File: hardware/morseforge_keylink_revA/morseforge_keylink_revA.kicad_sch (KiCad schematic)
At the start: 28 parts, among them J1 USB_C_Receptacle_USB2.0_14P, J2 Conn_01x02_Socket, Q1 Q_NPN_BCE, SW1 SW_SPST, SW2 SW_Push, SW3 SW_Push, U1 MCP73831-2-MC, U2 LDO40LPU33RY, U3 CP2102N-Axx-xQFN20

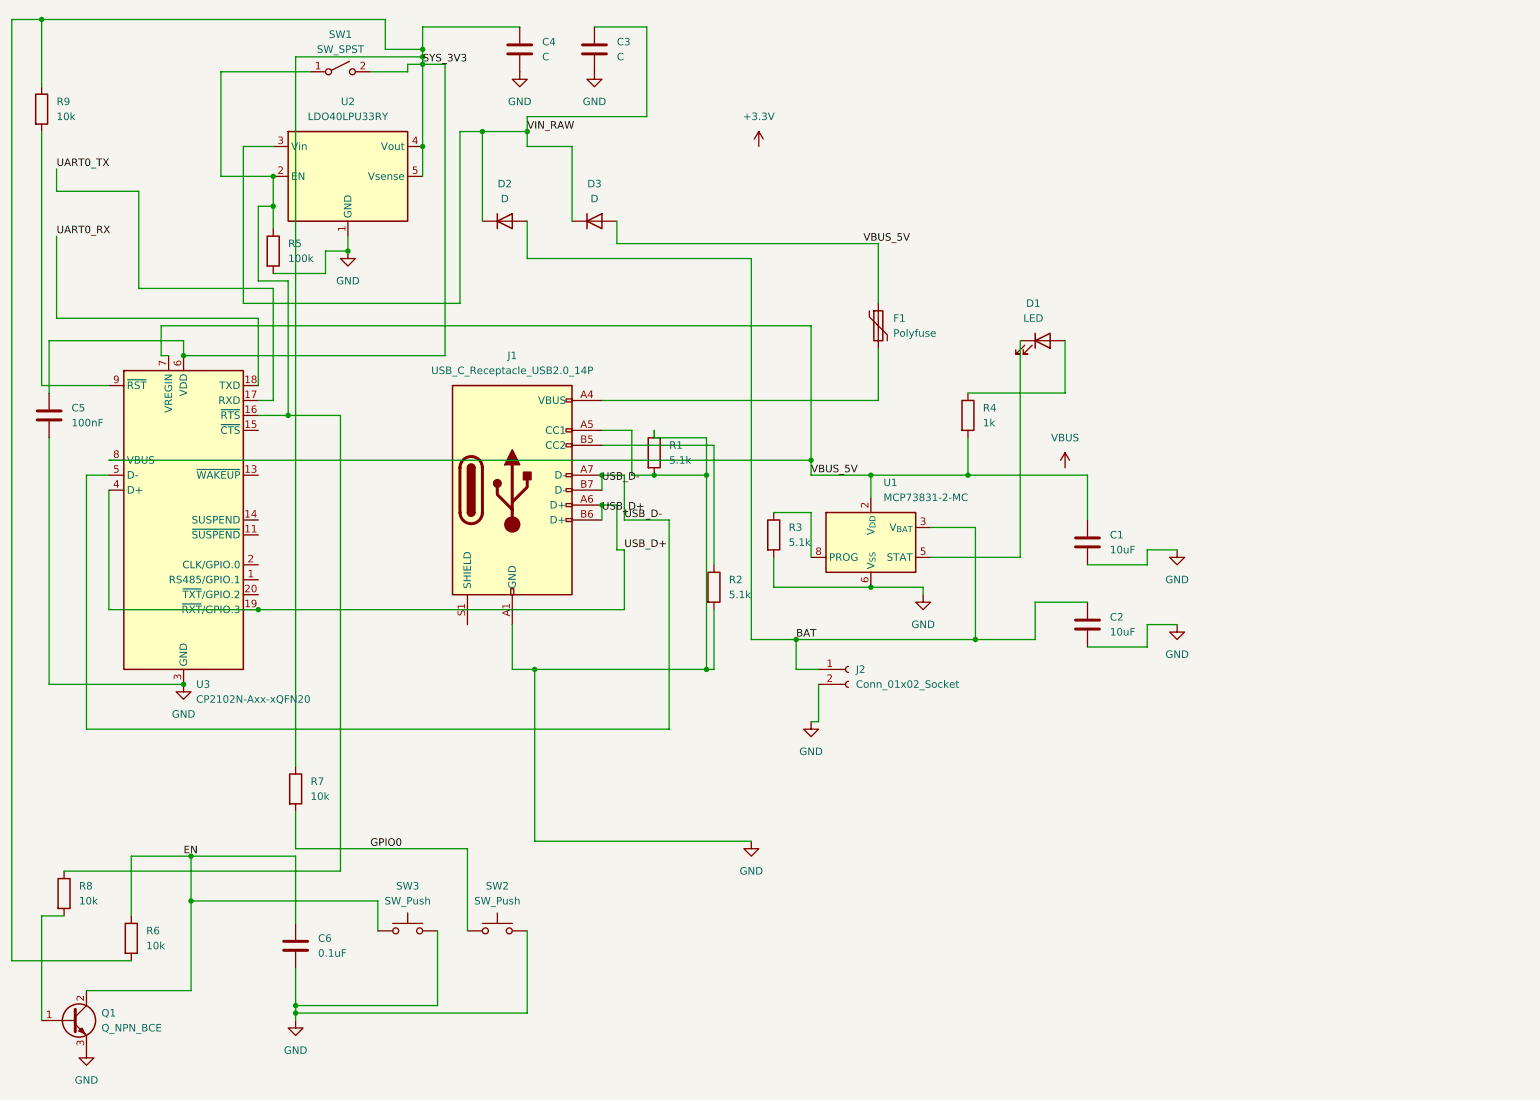
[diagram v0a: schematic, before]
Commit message: Adding in esp32
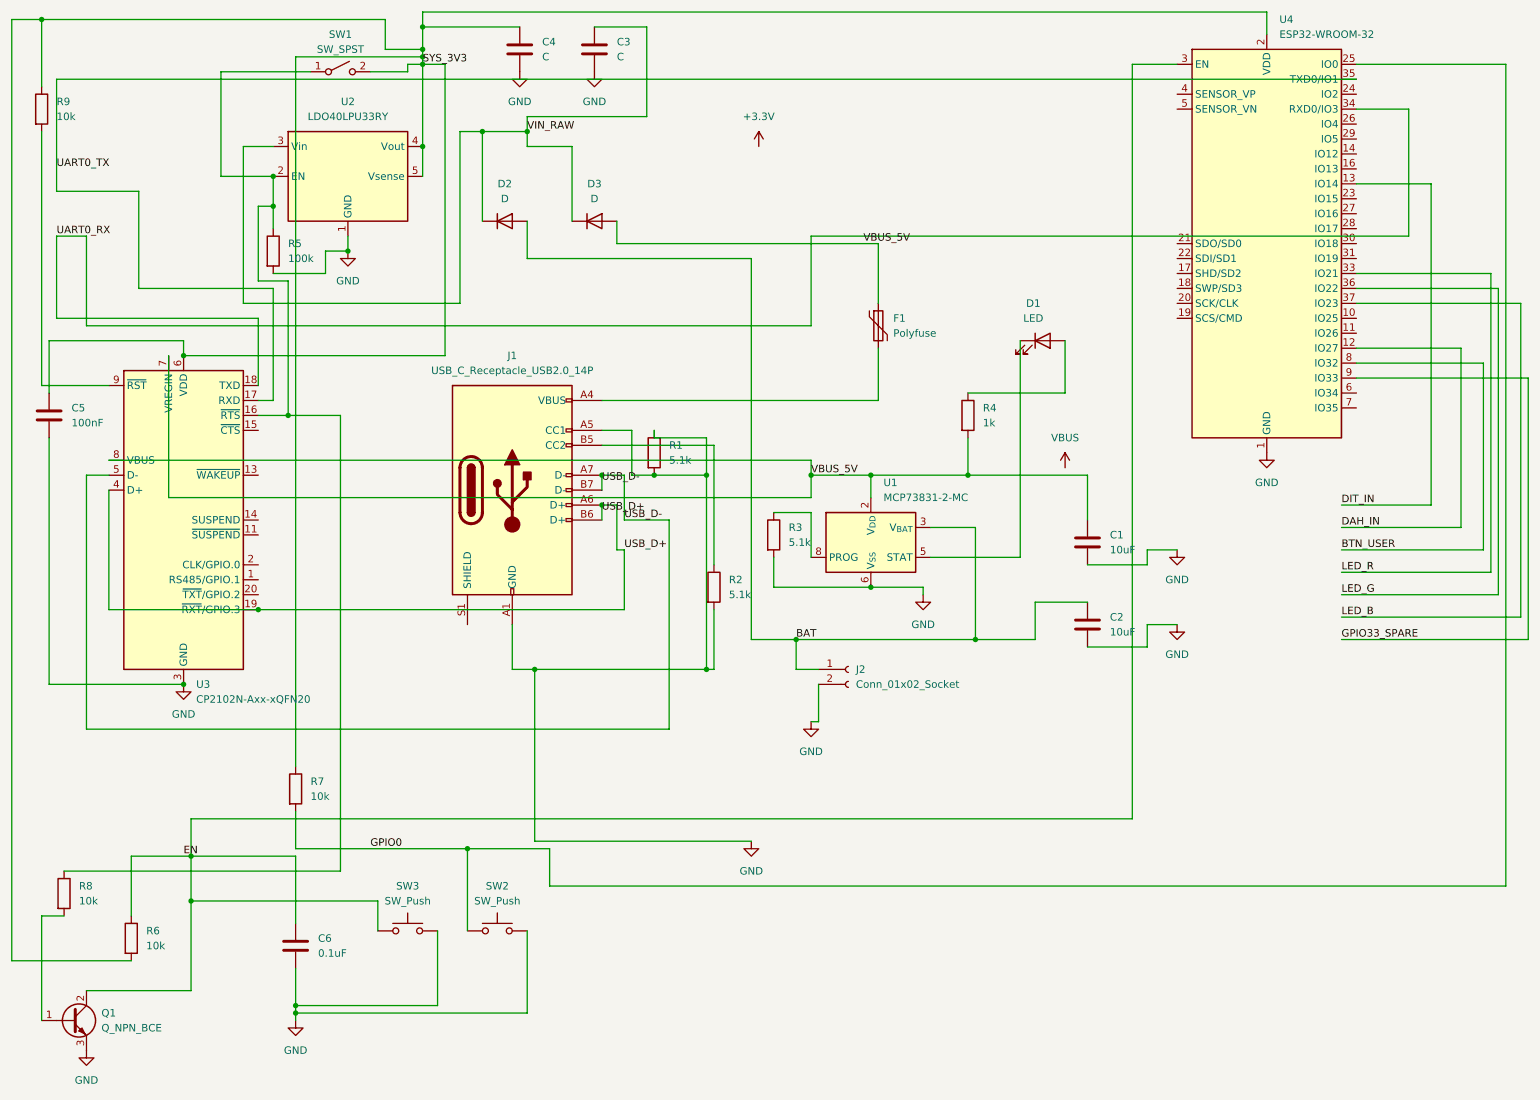
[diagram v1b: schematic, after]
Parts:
- added U4: ESP32-WROOM-32, RF_Module:ESP32-WROOM-32, symbol RF_Module:ESP32-WROOM-32
- U3: footprint Package_DFN_QFN:SiliconLabs_QFN-20-1EP_3x3mm_P0.5mm -> Package_DFN_QFN:QFN-20-1EP_3x3mm_P0.45mm_EP1.6x1.6mm
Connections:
- net EN: now also U4.3 (EN)
- net GND: now also U4.1 (GND), U4.15 (GND), U4.38 (GND), U4.39 (GND)
- net GPIO0: now also U4.25 (IO0)
- net SYS_3V3: now also U4.2 (VDD)
- net UART0_RX: now also U4.34 (RXD0/IO3)
- net UART0_TX: now also U4.35 (TXD0/IO1)
- new net BTN_USER: U4.8 (IO32)
- new net DAH_IN: U4.12 (IO27)
- new net DIT_IN: U4.13 (IO14)
- new net GPIO33_SPARE: U4.9 (IO33)
- new net LED_B: U4.37 (IO23)
- new net LED_G: U4.36 (IO22)
- new net LED_R: U4.33 (IO21)
